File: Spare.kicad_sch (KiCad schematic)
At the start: 9 parts, among them U11 74LS06, U12 74LS00, U13 74LS74, U19 74HCT74, U20 74LS74, U21 74LS14, U22 74LS06, U4 74LS86, U7 74LS32

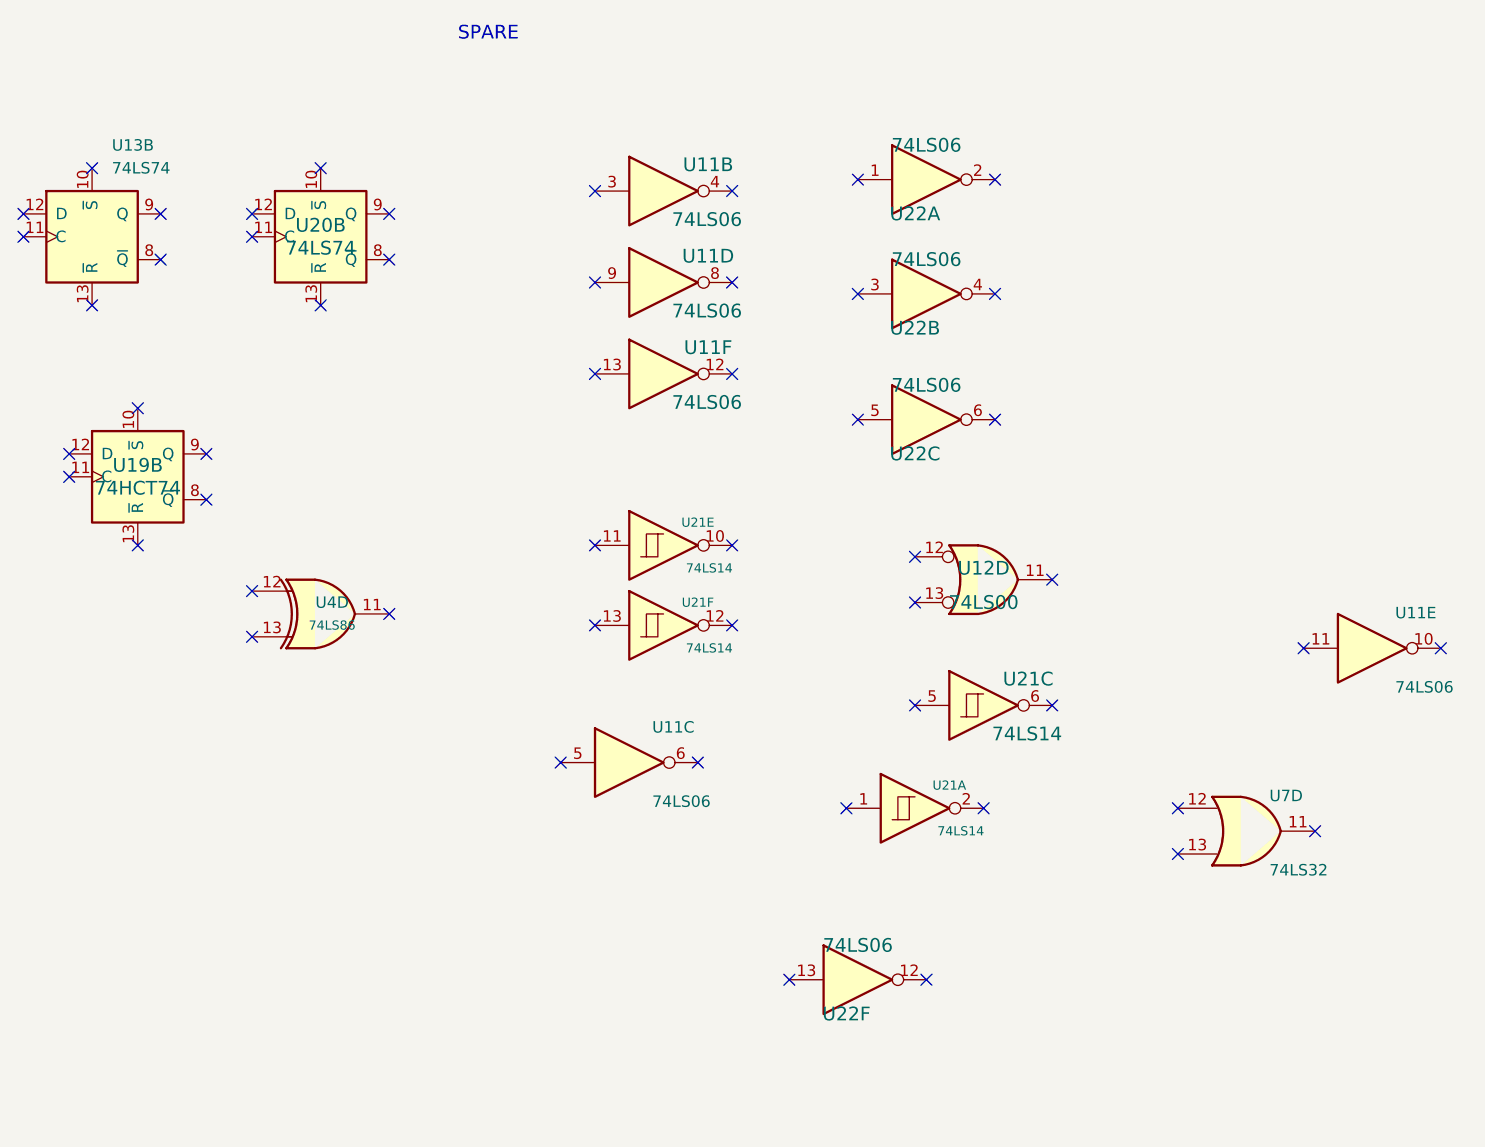
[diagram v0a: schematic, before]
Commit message: Schematic in progress
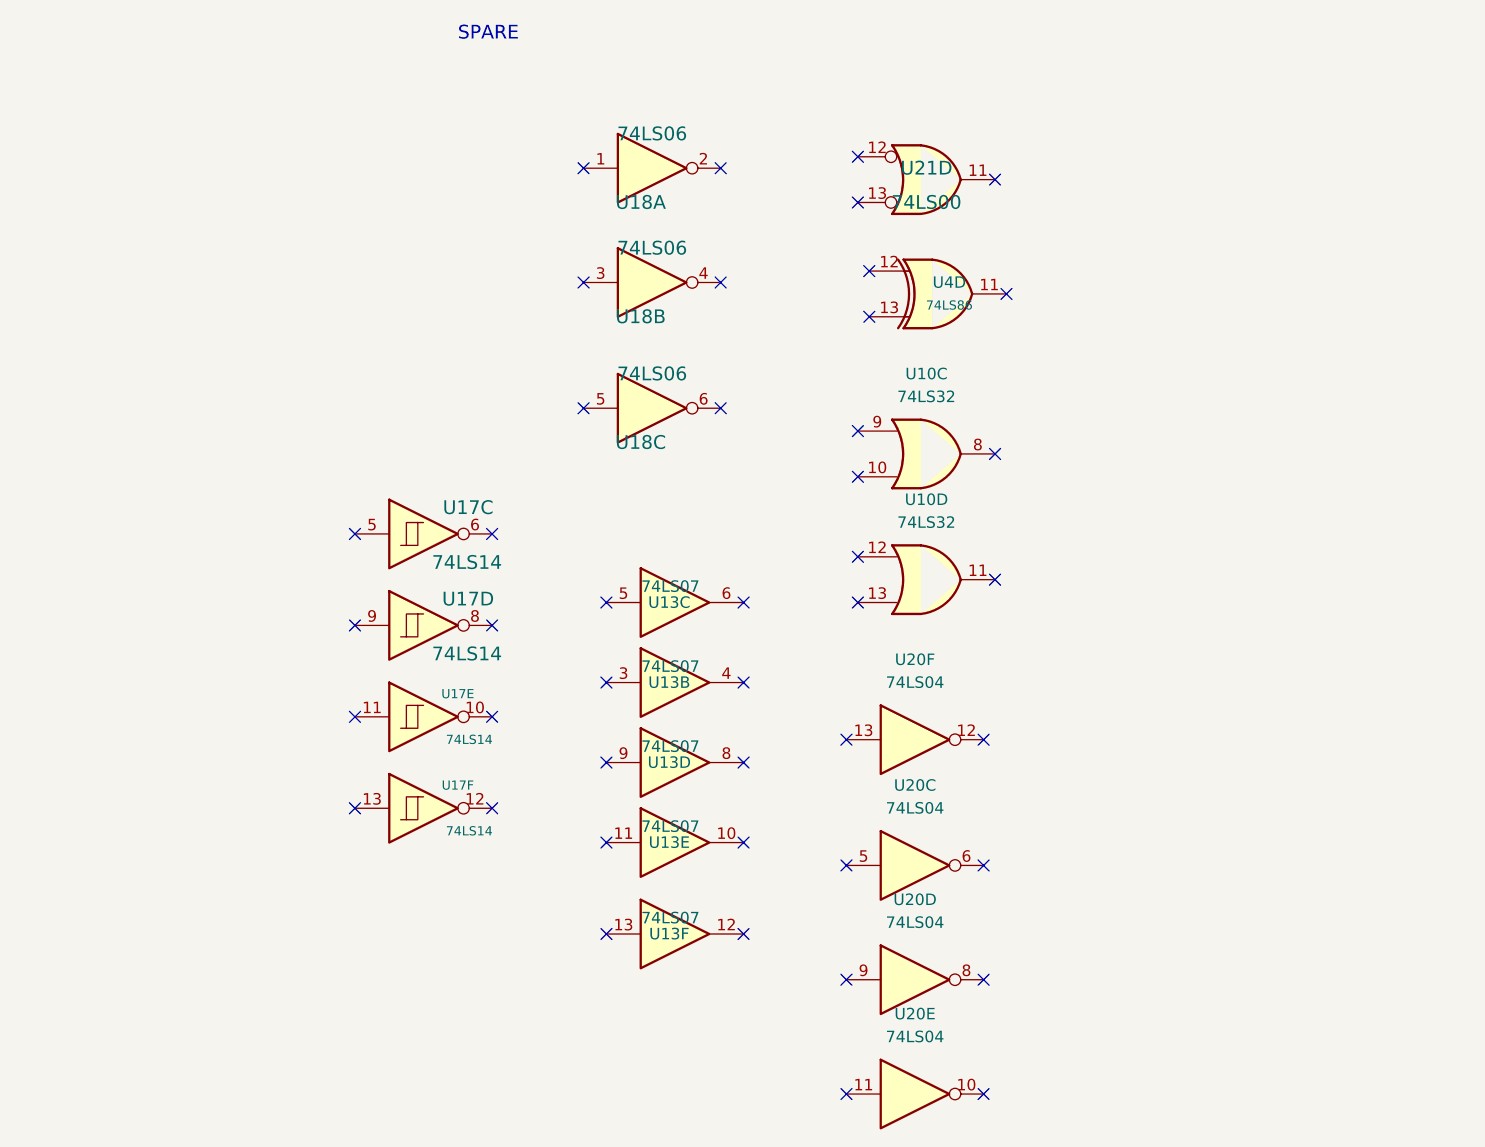
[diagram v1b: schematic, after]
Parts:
- removed U11: 74LS06, DIP-14__300, symbol 74xx:74LS06
- removed U13: 74LS74, symbol 74xx:74LS74
- removed U19: 74HCT74, DIP-14__300, symbol 74xx:74LS74
- removed U20: 74LS74, DIP-14__300, symbol 74xx:74LS74
- removed unit 1 of U21
- removed unit 6 of U22
- removed U7: 74LS32, DIP-14__300, symbol 74xx:74LS32
- added U10: 74LS32, Package_DIP:DIP-14_W7.62mm_Socket_LongPads, symbol 74xx:74LS32
- added U13: 74LS07, Package_DIP:DIP-14_W7.62mm_Socket_LongPads, symbol 74xx:74LS07
- added unit 4 of U17
- added U20: 74LS04, Package_DIP:DIP-14_W7.62mm_Socket_LongPads, symbol 74xx:74LS04
- U17: renamed from U21; footprint DIP-14__300 -> Package_DIP:DIP-14_W7.62mm_Socket_LongPads
- U18: renamed from U22; footprint DIP-14__300 -> Package_DIP:DIP-14_W7.62mm_Socket_LongPads
- U21: renamed from U12; footprint DIP-14__300 -> Package_DIP:DIP-14_W7.62mm_Socket_LongPads
- U4: footprint DIP-14__300 -> Package_DIP:DIP-14_W7.62mm_Socket_LongPads
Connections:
- no-connect marks 53 -> 44
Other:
- company: N8VEM Users Group -> (none)
- title: 6809 and 6502 ATX and 6U -> 6809PC
- moved on the sheet: U17C, U17E, U17F, U18A, U18B, U18C, U21D, U4D
